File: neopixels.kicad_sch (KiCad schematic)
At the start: 4 parts, among them J14 Conn_01x03_Pin, J15 Conn_01x02_Pin, J3 Conn_01x03_Pin

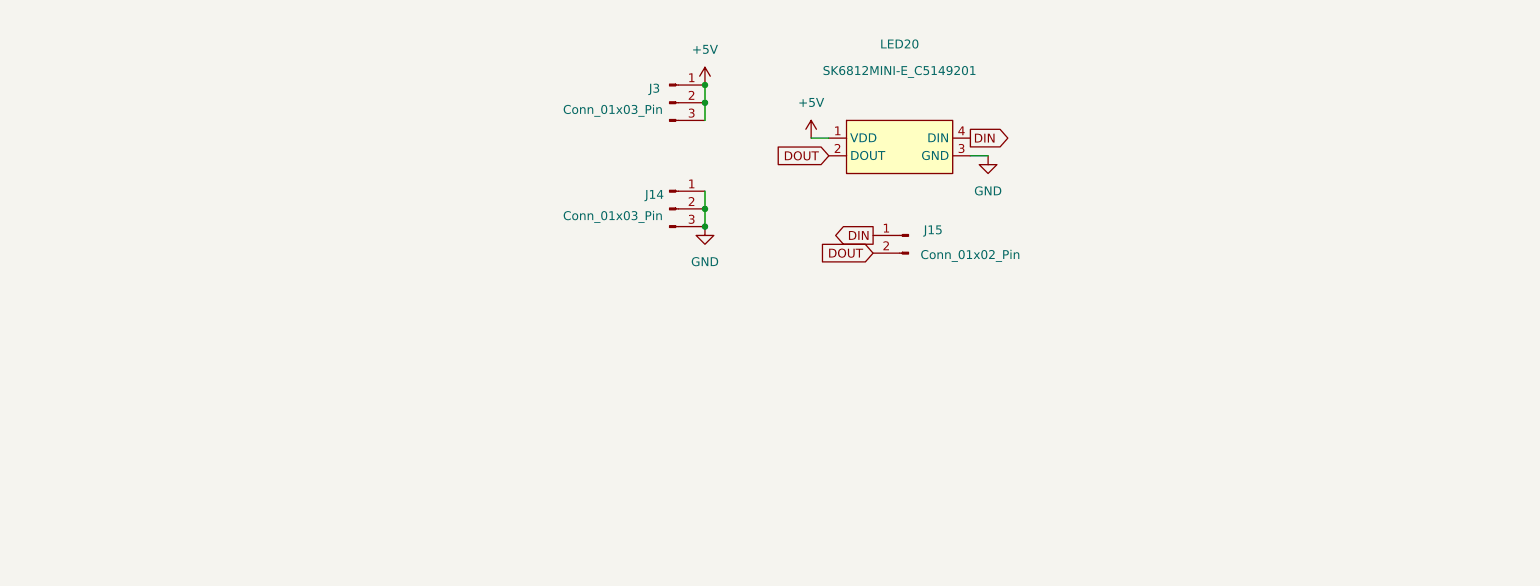
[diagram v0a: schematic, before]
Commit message: finished schematic yay!! now onto pcb routing :fire:
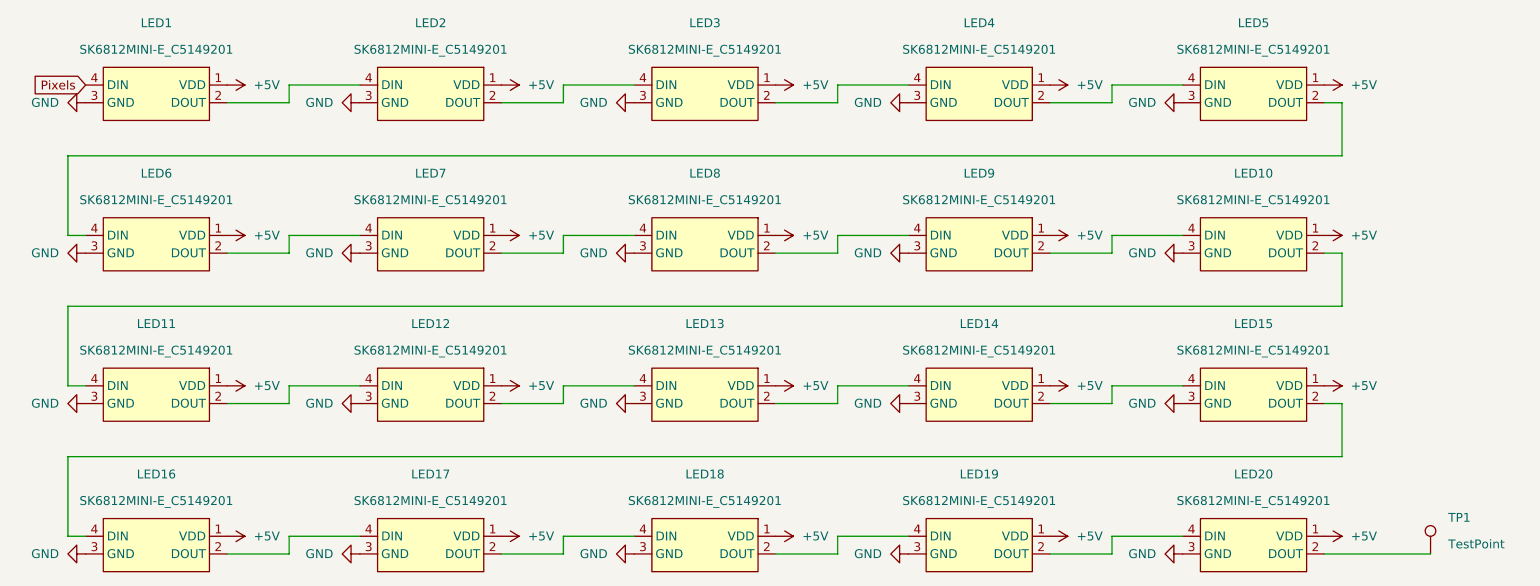
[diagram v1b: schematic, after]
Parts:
- removed J14, J3: Conn_01x03_Pin, symbol Connector:Conn_01x03_Pin
- removed J15: Conn_01x02_Pin, symbol Connector:Conn_01x02_Pin
- removed LED20: SK6812MINI-E_C5149201, easyeda2kicad:LED-SMD_L3.2-W2.8-LS5.9_SK6812MINI-E, symbol EasyEDA:SK6812MINI-E_C5149201
- added LED1, LED10, LED11, LED12, LED13, LED14, LED15, LED16, LED17, LED18, LED19, LED2, LED20, LED3, LED4, LED5, LED6, LED7, LED8, LED9: SK6812MINI-E_C5149201, easyeda2kicad:LED-SMD_L3.2-W2.8-LS5.9_SK6812MINI-E, symbol easyeda2kicad:SK6812MINI-E_C5149201
- added TP1: TestPoint, TestPoint:TestPoint_Pad_D2.5mm, symbol Connector:TestPoint
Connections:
- net +5V: now also LED1.1 (VDD), LED10.1 (VDD), LED11.1 (VDD), LED12.1 (VDD), LED13.1 (VDD), LED14.1 (VDD), LED15.1 (VDD), LED16.1 (VDD), LED17.1 (VDD), LED18.1 (VDD), LED19.1 (VDD), LED2.1 (VDD), LED20.1 (VDD), LED3.1 (VDD), LED4.1 (VDD), LED5.1 (VDD), LED6.1 (VDD), LED7.1 (VDD), LED8.1 (VDD), LED9.1 (VDD)
- net GND: now also LED1.3 (GND), LED10.3 (GND), LED11.3 (GND), LED12.3 (GND), LED13.3 (GND), LED14.3 (GND), LED15.3 (GND), LED16.3 (GND), LED17.3 (GND), LED18.3 (GND), LED19.3 (GND), LED2.3 (GND), LED20.3 (GND), LED3.3 (GND), LED4.3 (GND), LED5.3 (GND), LED6.3 (GND), LED7.3 (GND), LED8.3 (GND), LED9.3 (GND)
- new net: LED12.2 (DOUT), LED13.4 (DIN)
- new net: LED11.2 (DOUT), LED12.4 (DIN)
- new net: LED4.2 (DOUT), LED5.4 (DIN)
- new net: LED3.2 (DOUT), LED4.4 (DIN)
- new net: LED15.2 (DOUT), LED16.4 (DIN)
- new net: LED14.2 (DOUT), LED15.4 (DIN)
- new net: LED8.2 (DOUT), LED9.4 (DIN)
- new net: LED7.2 (DOUT), LED8.4 (DIN)
- new net: LED18.2 (DOUT), LED19.4 (DIN)
- new net: LED17.2 (DOUT), LED18.4 (DIN)
- new net: LED20.2 (DOUT), TP1.1
- new net: LED2.2 (DOUT), LED3.4 (DIN)
- new net: LED13.2 (DOUT), LED14.4 (DIN)
- new net: LED1.2 (DOUT), LED2.4 (DIN)
- new net: LED10.2 (DOUT), LED11.4 (DIN)
- new net: LED6.2 (DOUT), LED7.4 (DIN)
- new net: LED5.2 (DOUT), LED6.4 (DIN)
- new net: LED10.4 (DIN), LED9.2 (DOUT)
- new net: LED19.2 (DOUT), LED20.4 (DIN)
- new net: LED16.2 (DOUT), LED17.4 (DIN)
- new net Pixels: LED1.4 (DIN)

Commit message: made huge progress today, finished wiring up the rp2040, finished one usb a and usb c layout :fire::fire::fire:
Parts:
- LED1, LED10, LED11, LED12, LED13, LED14, LED15, LED16, LED17, LED18, LED19, LED2, LED20, LED3, LED4, LED5, LED6, LED7, LED8, LED9: footprint easyeda2kicad:LED-SMD_L3.2-W2.8-LS5.9_SK6812MINI-E -> Keebio-Parts:SK6812-MINI-E
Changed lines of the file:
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@@
 			)
 		)
-		(property "Footprint" "easyeda2kicad:LED-SMD_L3.2-W2.8-LS5.9_SK6812MINI-E"
+		(property "Footprint" "Keebio-Parts:SK6812-MINI-E"
 			(at 116.84 93.98 0)
 			(effects
@@
 			)
 		)
-		(property "Footprint" "easyeda2kicad:LED-SMD_L3.2-W2.8-LS5.9_SK6812MINI-E"
+		(property "Footprint" "Keebio-Parts:SK6812-MINI-E"
 			(at 195.58 50.8 0)
 			(effects
@@
 			)
 		)
-		(property "Footprint" "easyeda2kicad:LED-SMD_L3.2-W2.8-LS5.9_SK6812MINI-E"
+		(property "Footprint" "Keebio-Parts:SK6812-MINI-E"
 			(at 234.95 93.98 0)
 			(effects
@@
 			)
 		)
-		(property "Footprint" "easyeda2kicad:LED-SMD_L3.2-W2.8-LS5.9_SK6812MINI-E"
+		(property "Footprint" "Keebio-Parts:SK6812-MINI-E"
 			(at 156.21 72.39 0)
 			(effects
@@
 			)
 		)
-		(property "Footprint" "easyeda2kicad:LED-SMD_L3.2-W2.8-LS5.9_SK6812MINI-E"
+		(property "Footprint" "Keebio-Parts:SK6812-MINI-E"
 			(at 156.21 115.57 0)
 			(effects
@@
 			)
 		)
-		(property "Footprint" "easyeda2kicad:LED-SMD_L3.2-W2.8-LS5.9_SK6812MINI-E"
+		(property "Footprint" "Keebio-Parts:SK6812-MINI-E"
 			(at 156.21 50.8 0)
 			(effects
@@
 			)
 		)
-		(property "Footprint" "easyeda2kicad:LED-SMD_L3.2-W2.8-LS5.9_SK6812MINI-E"
+		(property "Footprint" "Keebio-Parts:SK6812-MINI-E"
 			(at 156.21 93.98 0)
 			(effects
@@
 			)
 		)
-		(property "Footprint" "easyeda2kicad:LED-SMD_L3.2-W2.8-LS5.9_SK6812MINI-E"
+		(property "Footprint" "Keebio-Parts:SK6812-MINI-E"
 			(at 195.58 93.98 0)
 			(effects
@@
 			)
 		)
-		(property "Footprint" "easyeda2kicad:LED-SMD_L3.2-W2.8-LS5.9_SK6812MINI-E"
+		(property "Footprint" "Keebio-Parts:SK6812-MINI-E"
 			(at 77.47 50.8 0)
 			(effects
@@
 			)
 		)
-		(property "Footprint" "easyeda2kicad:LED-SMD_L3.2-W2.8-LS5.9_SK6812MINI-E"
+		(property "Footprint" "Keebio-Parts:SK6812-MINI-E"
 			(at 77.47 93.98 0)
 			(effects
@@
 			)
 		)
-		(property "Footprint" "easyeda2kicad:LED-SMD_L3.2-W2.8-LS5.9_SK6812MINI-E"
+		(property "Footprint" "Keebio-Parts:SK6812-MINI-E"
 			(at 77.47 72.39 0)
 			(effects
@@
 			)
 		)
-		(property "Footprint" "easyeda2kicad:LED-SMD_L3.2-W2.8-LS5.9_SK6812MINI-E"
+		(property "Footprint" "Keebio-Parts:SK6812-MINI-E"
 			(at 116.84 72.39 0)
 			(effects
@@
 			)
 		)
-		(property "Footprint" "easyeda2kicad:LED-SMD_L3.2-W2.8-LS5.9_SK6812MINI-E"
+		(property "Footprint" "Keebio-Parts:SK6812-MINI-E"
 			(at 234.95 72.39 0)
 			(effects
@@
 			)
 		)
-		(property "Footprint" "easyeda2kicad:LED-SMD_L3.2-W2.8-LS5.9_SK6812MINI-E"
+		(property "Footprint" "Keebio-Parts:SK6812-MINI-E"
 			(at 116.84 50.8 0)
 			(effects
@@
 			)
 		)
-		(property "Footprint" "easyeda2kicad:LED-SMD_L3.2-W2.8-LS5.9_SK6812MINI-E"
+		(property "Footprint" "Keebio-Parts:SK6812-MINI-E"
 			(at 234.95 115.57 0)
 			(effects
@@
 			)
 		)
-		(property "Footprint" "easyeda2kicad:LED-SMD_L3.2-W2.8-LS5.9_SK6812MINI-E"
+		(property "Footprint" "Keebio-Parts:SK6812-MINI-E"
 			(at 195.58 72.39 0)
 			(effects
@@
 			)
 		)
-		(property "Footprint" "easyeda2kicad:LED-SMD_L3.2-W2.8-LS5.9_SK6812MINI-E"
+		(property "Footprint" "Keebio-Parts:SK6812-MINI-E"
 			(at 234.95 50.8 0)
 			(effects
@@
 			)
 		)
-		(property "Footprint" "easyeda2kicad:LED-SMD_L3.2-W2.8-LS5.9_SK6812MINI-E"
+		(property "Footprint" "Keebio-Parts:SK6812-MINI-E"
 			(at 195.58 115.57 0)
 			(effects
@@
 			)
 		)
-		(property "Footprint" "easyeda2kicad:LED-SMD_L3.2-W2.8-LS5.9_SK6812MINI-E"
+		(property "Footprint" "Keebio-Parts:SK6812-MINI-E"
 			(at 77.47 115.57 0)
 			(effects
@@
 			)
 		)
-		(property "Footprint" "easyeda2kicad:LED-SMD_L3.2-W2.8-LS5.9_SK6812MINI-E"
+		(property "Footprint" "Keebio-Parts:SK6812-MINI-E"
 			(at 116.84 115.57 0)
 			(effects
